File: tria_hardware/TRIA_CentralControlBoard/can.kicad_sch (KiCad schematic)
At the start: 5 parts, among them J5 resistor_enable, U9 MCP2562-E-P

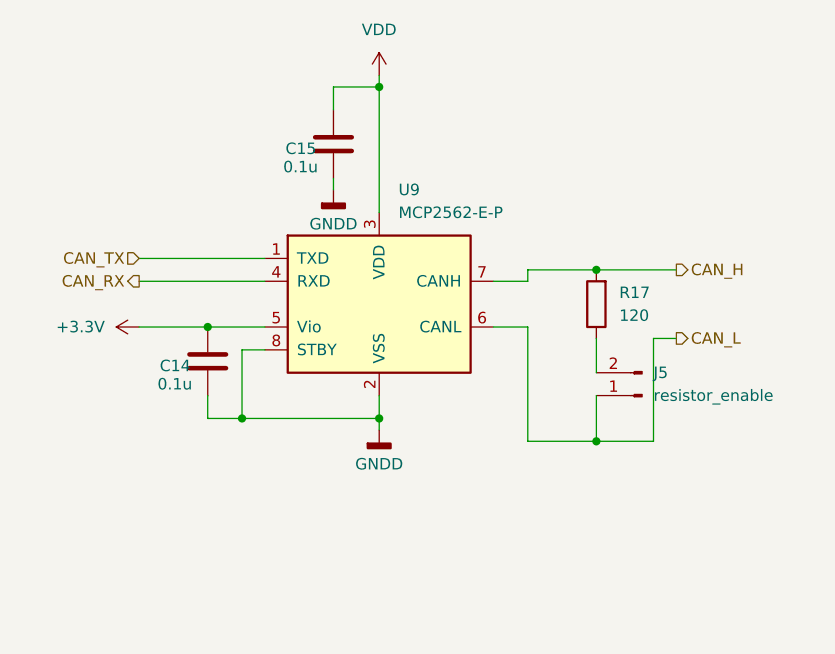
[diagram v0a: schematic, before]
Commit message: [update] 基板データのアップデート
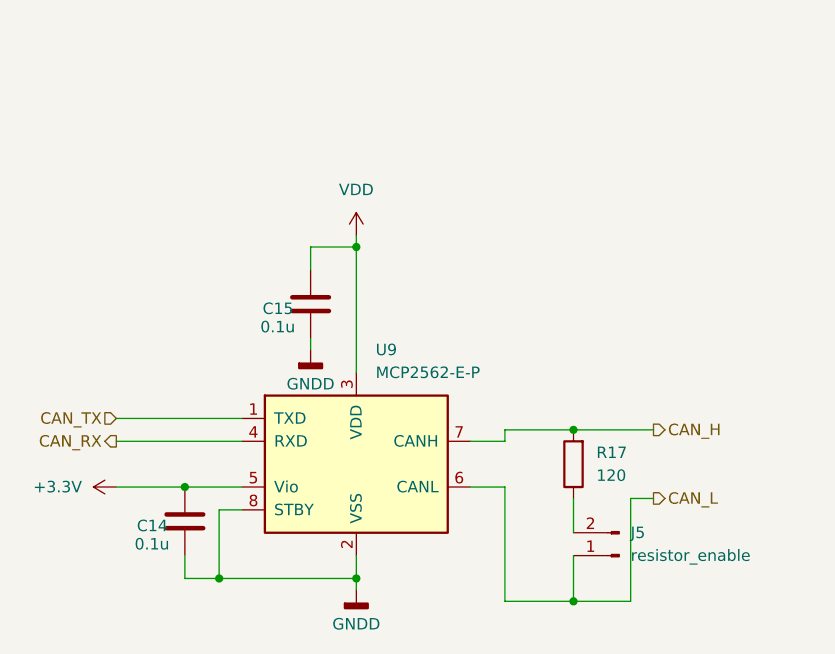
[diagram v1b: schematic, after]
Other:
- moved on the sheet: C14, C15, J5, R17, U9
